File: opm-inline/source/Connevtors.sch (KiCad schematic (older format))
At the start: 17 parts, among them U201 Metz_31330102, U202 Metz_31349102, U203 Metz_31330103, U204 Metz_31349103

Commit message: update libs
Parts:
- C201, C202: LCSC (none) -> C340711; manf_num (none) -> UCD2A221MNQ1MS
- U201: symbol TMC6100-EVAL-v1.2-rescue:Metz_31330102-Conector_library-TMC6100-EVAL-v1.2-rescue -> opm-cache:Conector_library_Metz_31330102
- U202: symbol TMC6100-EVAL-v1.2-rescue:Metz_31349102-Conector_library-TMC6100-EVAL-v1.2-rescue -> opm-cache:Conector_library_Metz_31349102
- U203: symbol TMC6100-EVAL-v1.2-rescue:Metz_31330103-Conector_library-TMC6100-EVAL-v1.2-rescue -> opm-cache:Conector_library_Metz_31330103
- U204: symbol TMC6100-EVAL-v1.2-rescue:Metz_31349103-Conector_library-TMC6100-EVAL-v1.2-rescue -> opm-cache:Conector_library_Metz_31349103
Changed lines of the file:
@@
 $EndDescr
 $Comp
-L TMC6100-EVAL-v1.2-rescue:Metz_31330102-Conector_library-TMC6100-EVAL-v1.2-rescue U201
+L opm-cache:Conector_library_Metz_31330102 U201
 U 1 1 5C0100EA
 P 1550 1250
@@
 $EndComp
 $Comp
-L TMC6100-EVAL-v1.2-rescue:Metz_31349102-Conector_library-TMC6100-EVAL-v1.2-rescue U202
+L opm-cache:Conector_library_Metz_31349102 U202
 U 1 1 5C59EB06
 P 1000 1250
@@
 F 2 "Capacitor_THT:CP_Radial_D12.5mm_P5.00mm" V 2600 1450 39  0001 C CNN
 F 3 "~" H 2400 1450 39  0001 C CNN
+F 4 "C340711" V 2400 1450 50  0001 C CNN "LCSC"
+F 5 "UCD2A221MNQ1MS" V 2400 1450 50  0001 C CNN "manf_num"
 	1    2400 1450
 	1    0    0    -1
@@
 F 2 "Capacitor_THT:CP_Radial_D12.5mm_P5.00mm" H 2900 1450 39  0001 C CNN
 F 3 "~" H 2900 1450 39  0001 C CNN
+F 4 "C340711" V 2900 1450 50  0001 C CNN "LCSC"
+F 5 "UCD2A221MNQ1MS" V 2900 1450 50  0001 C CNN "manf_num"
 	1    2900 1450
 	1    0    0    -1
@@
 Connection ~ 2900 1700
 $Comp
-L TMC6100-EVAL-v1.2-rescue:Metz_31330103-Conector_library-TMC6100-EVAL-v1.2-rescue U203
+L opm-cache:Conector_library_Metz_31330103 U203
 U 1 1 5D65AFA7
 P 2450 2350
@@
 	3450 750  650  750
 $Comp
-L TMC6100-EVAL-v1.2-rescue:Metz_31349103-Conector_library-TMC6100-EVAL-v1.2-rescue U204
+L opm-cache:Conector_library_Metz_31349103 U204
 U 1 1 5DA86CEE
 P 3000 2350

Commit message: update connectors
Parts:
- H201, H202, H203, H204: symbol TMC6100-EVAL-v1.2-rescue:MountingHole_Pad-Mechanical-TMC6100-EVAL-v1.2-rescue -> opm-cache:Mechanical_MountingHole_Pad
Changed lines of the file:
@@
 $EndComp
 $Comp
-L TMC6100-EVAL-v1.2-rescue:MountingHole_Pad-Mechanical-TMC6100-EVAL-v1.2-rescue H204
+L opm-cache:Mechanical_MountingHole_Pad H204
 U 1 1 5C3360CB
 P 3950 1700
@@
 $EndComp
 $Comp
-L TMC6100-EVAL-v1.2-rescue:MountingHole_Pad-Mechanical-TMC6100-EVAL-v1.2-rescue H203
+L opm-cache:Mechanical_MountingHole_Pad H203
 U 1 1 5C335E56
 P 3950 1500
@@
 $EndComp
 $Comp
-L TMC6100-EVAL-v1.2-rescue:MountingHole_Pad-Mechanical-TMC6100-EVAL-v1.2-rescue H202
+L opm-cache:Mechanical_MountingHole_Pad H202
 U 1 1 5C335D22
 P 3950 1300
@@
 $EndComp
 $Comp
-L TMC6100-EVAL-v1.2-rescue:MountingHole_Pad-Mechanical-TMC6100-EVAL-v1.2-rescue H201
+L opm-cache:Mechanical_MountingHole_Pad H201
 U 1 1 5C33535A
 P 3950 1100

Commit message: add fiducials
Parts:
- fid201, fid202, fid203: symbol TMC6100-EVAL-v1.0-rescue:fiducial-markings -> fiducual:fiducial-markings
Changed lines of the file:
@@
 	1750 1300 1650 1300
 $Comp
-L TMC6100-EVAL-v1.0-rescue:fiducial-markings fid201
+L fiducual:fiducial-markings fid201
 U 1 1 5C6BBB15
 P 4800 1050
@@
 $EndComp
 $Comp
-L TMC6100-EVAL-v1.0-rescue:fiducial-markings fid202
+L fiducual:fiducial-markings fid202
 U 1 1 5C6BC61F
 P 4800 1200
@@
 $EndComp
 $Comp
-L TMC6100-EVAL-v1.0-rescue:fiducial-markings fid203
+L fiducual:fiducial-markings fid203
 U 1 1 5C6BC9A9
 P 4800 1350

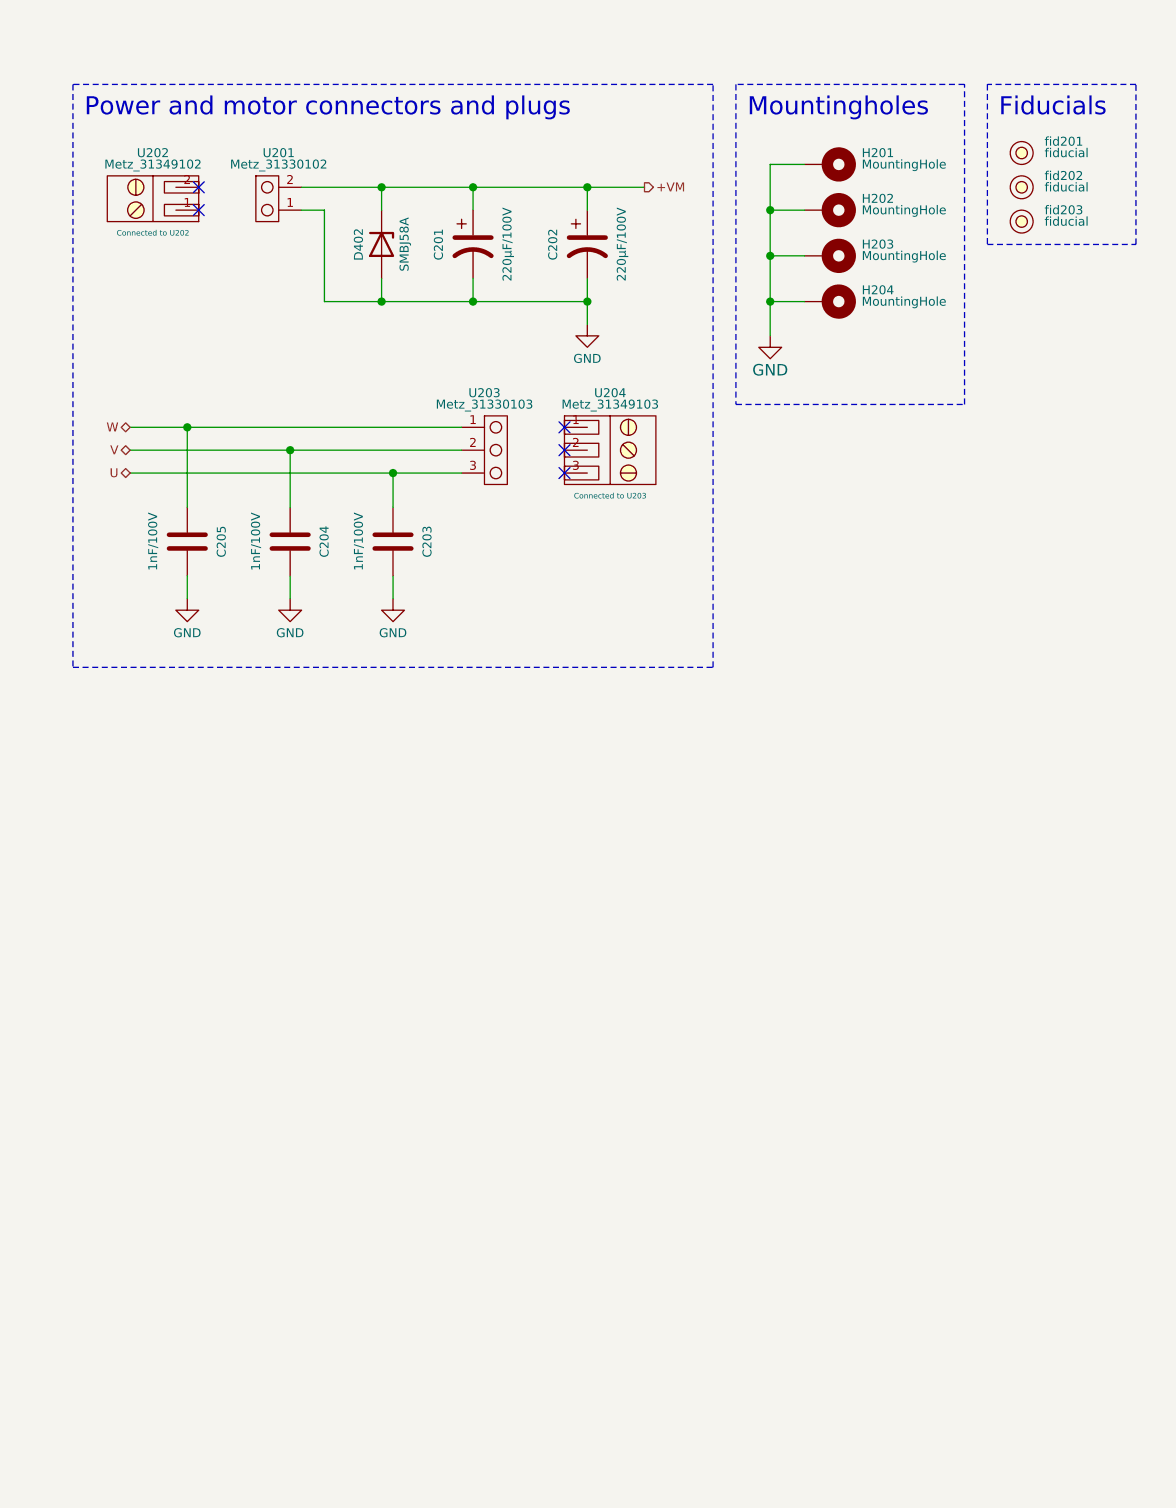
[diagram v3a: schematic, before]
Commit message: cleanup
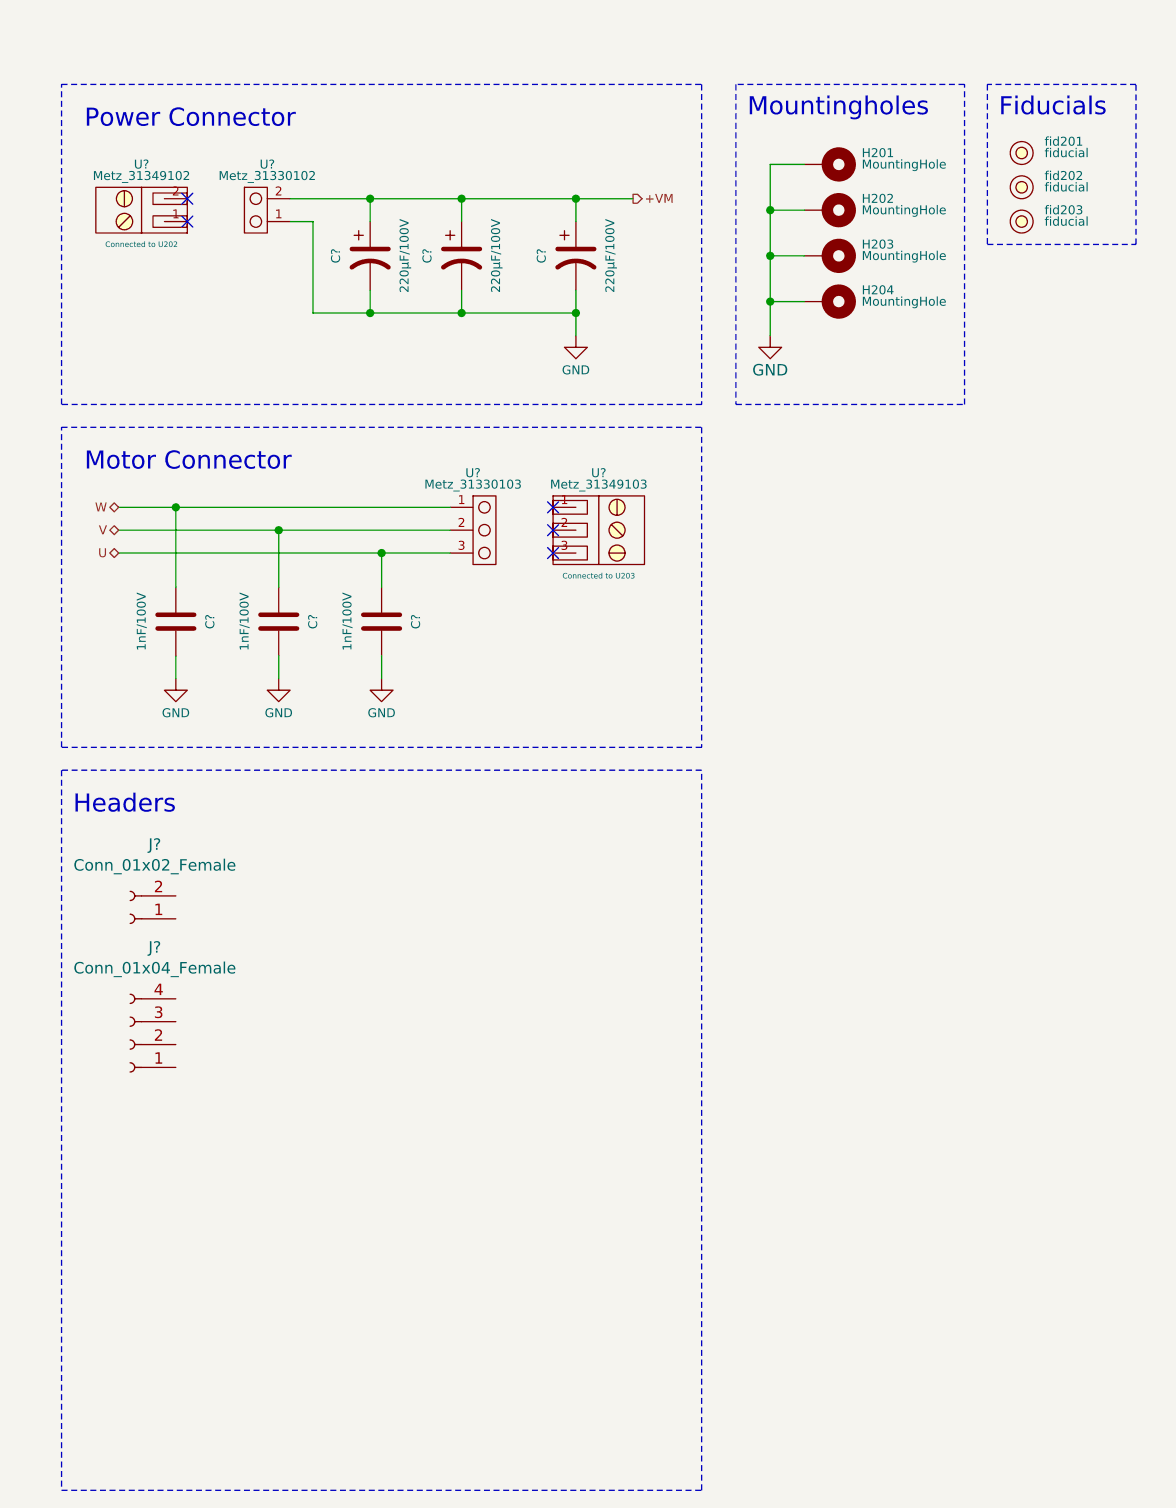
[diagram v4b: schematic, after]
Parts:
- removed C201, C202: 220μF/100V, Capacitor_THT:CP_Radial_D12.5mm_P5.00mm, symbol Device:CP1
- removed C203, C204, C205: 1nF/100V, Capacitor_SMD:C_0603_1608Metric, symbol Device:C
- removed D402: SMBJ58A, Diode_SMD:D_SMB, symbol Device:D_Zener
- removed U201: Metz_31330102, TerminalBlock_MetzConnect:TerminalBlock_MetzConnect_Type011_RT05502HBWC_1x02_P5.00mm_Horizontal, symbol opm-cache:Conector_library_Metz_31330102
- removed U202: Metz_31349102, symbol opm-cache:Conector_library_Metz_31349102
- removed U203: Metz_31330103, Connector_library:Metz_31330103, symbol opm-cache:Conector_library_Metz_31330103
- removed U204: Metz_31349103, symbol opm-cache:Conector_library_Metz_31349103
- added C? (x3): 1nF/100V, Capacitor_SMD:C_0603_1608Metric, symbol Device:C
- added C? (x3): 220μF/100V, Capacitor_THT:CP_Radial_D12.5mm_P5.00mm, symbol Device:CP1
- added J?: Conn_01x02_Female, symbol Connector:Conn_01x02_Female
- added J?: Conn_01x04_Female, symbol Connector:Conn_01x04_Female
- added U?: Metz_31330103, Connector_library:Metz_31330103, symbol opm-cache:Conector_library_Metz_31330103
- added U?: Metz_31349103, symbol opm-cache:Conector_library_Metz_31349103
- added U?: Metz_31330102, TerminalBlock_MetzConnect:TerminalBlock_MetzConnect_Type011_RT05502HBWC_1x02_P5.00mm_Horizontal, symbol opm-cache:Conector_library_Metz_31330102
- added U?: Metz_31349102, symbol opm-cache:Conector_library_Metz_31349102
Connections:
- net +VM: now also C?.1, C?.1, C?.1, U?.2
- net GND: now also C?.2, C?.2, C?.2, C?.2, C?.2, C?.2, U?.1
- net U: now also C?.1, U?.3
- net V: now also C?.1, U?.2
- net W: now also C?.1, U?.1
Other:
- note added: "Headers"
- note added: "Motor Connector"
- note added: "Power Connector"
- note removed: "Power and motor connectors and plugs"
